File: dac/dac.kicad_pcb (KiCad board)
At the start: 4 copper layers, 50 x 25 mm, 33 parts, among them J1 USB_B, J2 Conn_01x04_Pin, J3 Conn_01x04_Pin, U1 PCM2902, U2 SPX3819M5-L, Y1 12MHz

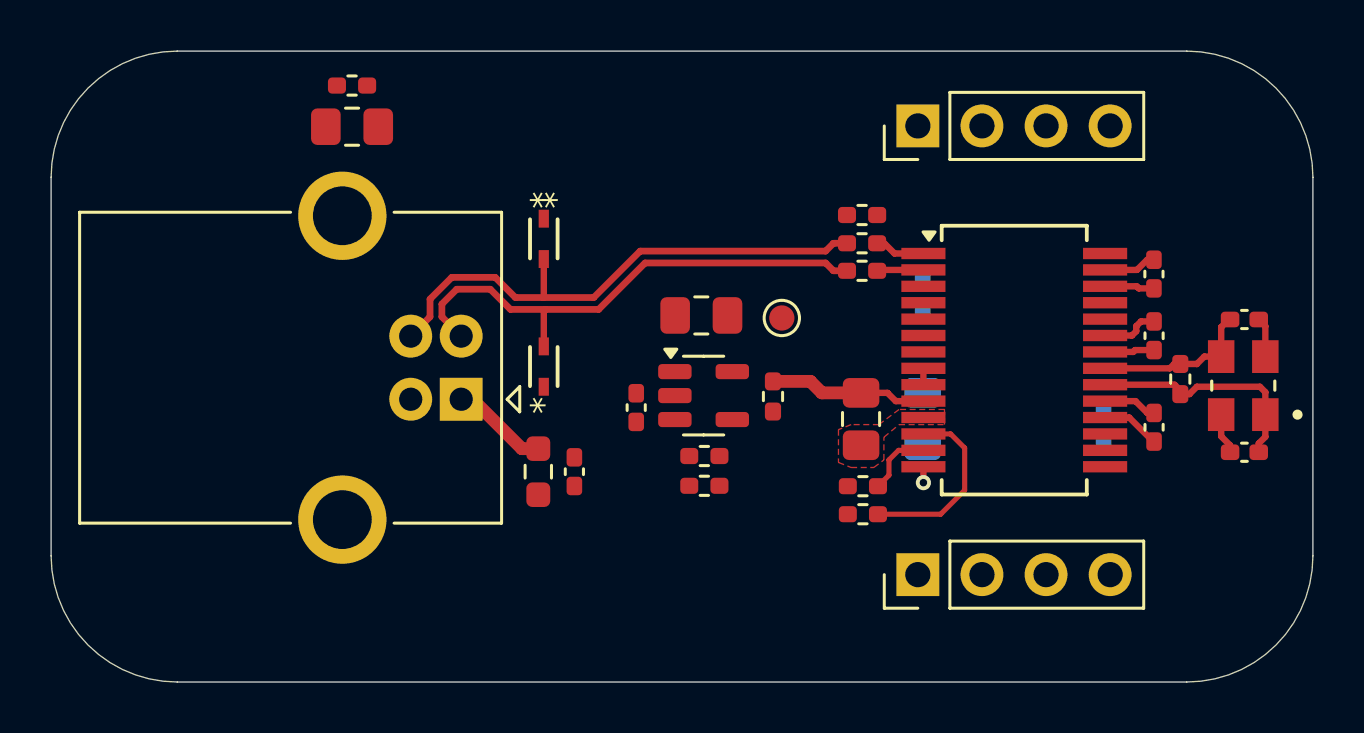
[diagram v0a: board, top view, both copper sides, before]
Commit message: layout is complete
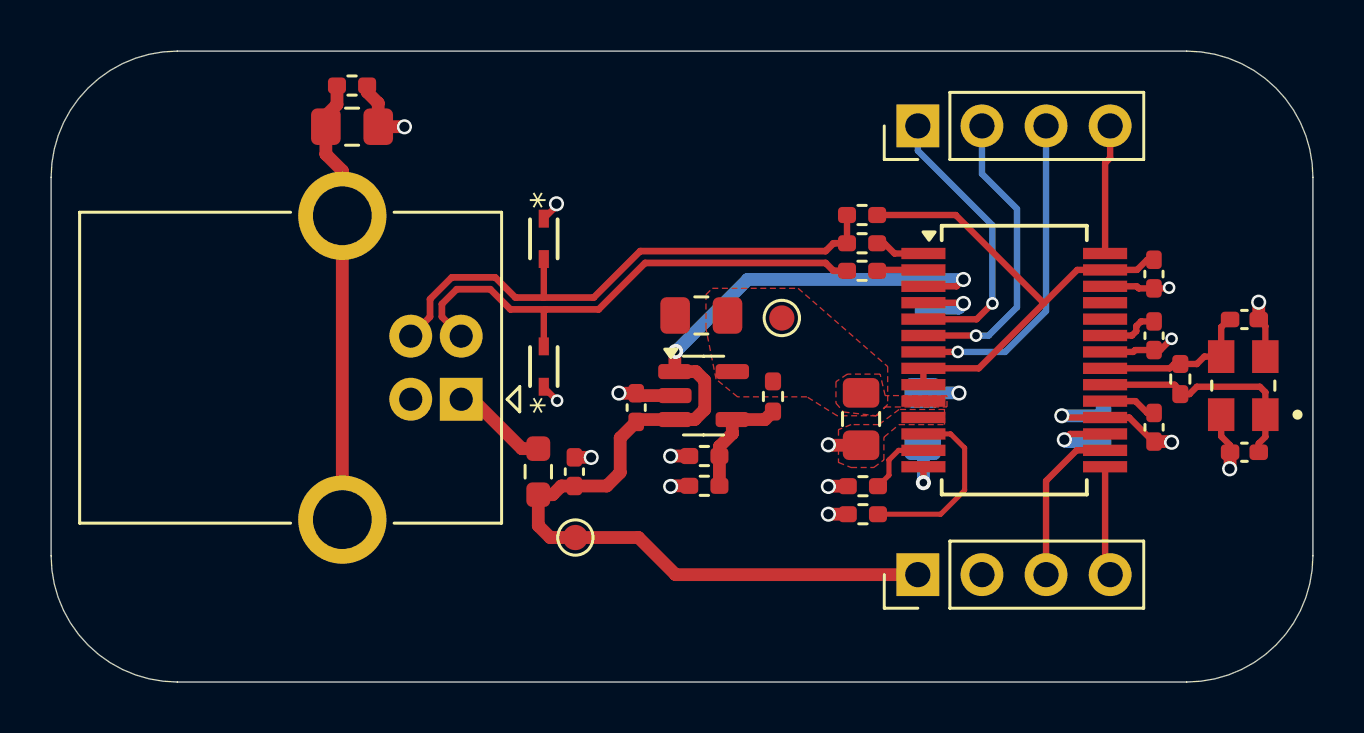
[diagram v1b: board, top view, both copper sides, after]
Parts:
- added TP2: TestPoint, TestPoint:TestPoint_Pad_D1.0mm, F.Cu at (85.8, 94.3)
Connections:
- J2 pad 1: unconnected-(J2-Pin_1-Pad1) -> VBUS
- J2 pad 2: unconnected-(J2-Pin_2-Pad2) -> GND
- J2 pad 3: unconnected-(J2-Pin_3-Pad3) -> /VOUTL
- J2 pad 4: unconnected-(J2-Pin_4-Pad4) -> /VOUTR
- J3 pad 1: unconnected-(J3-Pin_1-Pad1) -> /HID0
- J3 pad 2: unconnected-(J3-Pin_2-Pad2) -> /HID1
- J3 pad 3: unconnected-(J3-Pin_3-Pad3) -> /HID2
- J3 pad 4: unconnected-(J3-Pin_4-Pad4) -> /~{SSPND}
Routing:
- net VBUS: track 0.00 -> 43.4 mm, vias 0 -> 2
- net GND: track 9.49 -> 33.1 mm, vias 0 -> 18
- net CGND: track 0.00 -> 17.7 mm
- net VDDI: track 2.75 -> 19.6 mm
- net /HID2: track 0.00 -> 12.9 mm, vias 0 -> 1
- net /HID1: track 0.00 -> 11.9 mm, vias 0 -> 1
- net /HID0: track 0.00 -> 11.3 mm, vias 0 -> 1
- net /VOUTL: track 0.00 -> 6.56 mm
- net 3V7: track 6.28 -> 0.00 mm
- net /~{SSPND}: track 0.00 -> 5.14 mm
- net /ADJ: track 0.00 -> 4.59 mm
- net /VOUTR: track 0.00 -> 4.36 mm
- net /VCCP1I: track 0.00 -> 3.30 mm, vias 0 -> 1
- net /VCOM: track 0.63 -> 2.12 mm
- net /CONN_D+: track 21.4 -> 22.5 mm
- added copper zone on F.Cu, net 3V7
- added copper zone on In1.Cu, net GND
- added copper zone on In2.Cu, net GND
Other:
- board text removed: "teardrop here."
